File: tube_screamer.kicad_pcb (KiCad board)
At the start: 2 copper layers, 38 x 45 mm, 37 parts, among them Q1 BC817, U1 TL072

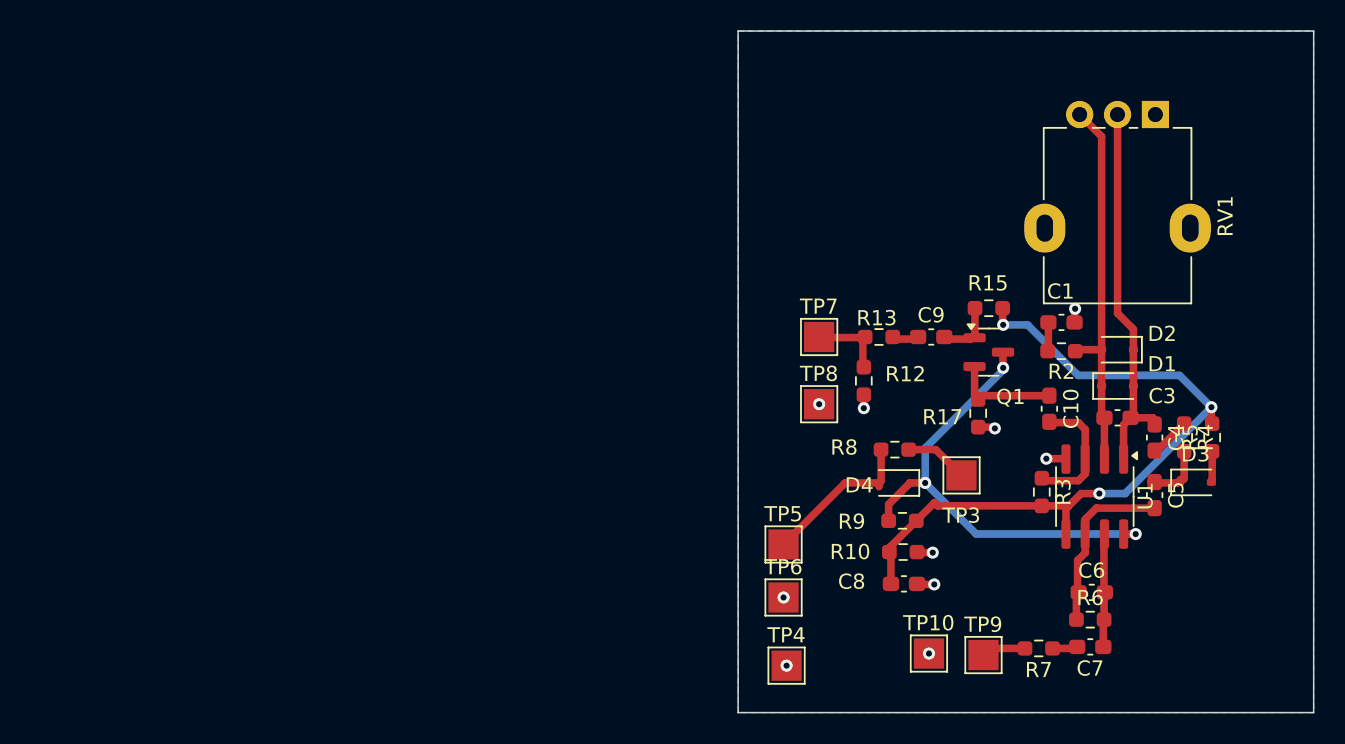
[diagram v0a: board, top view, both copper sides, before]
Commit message: Updated schematic
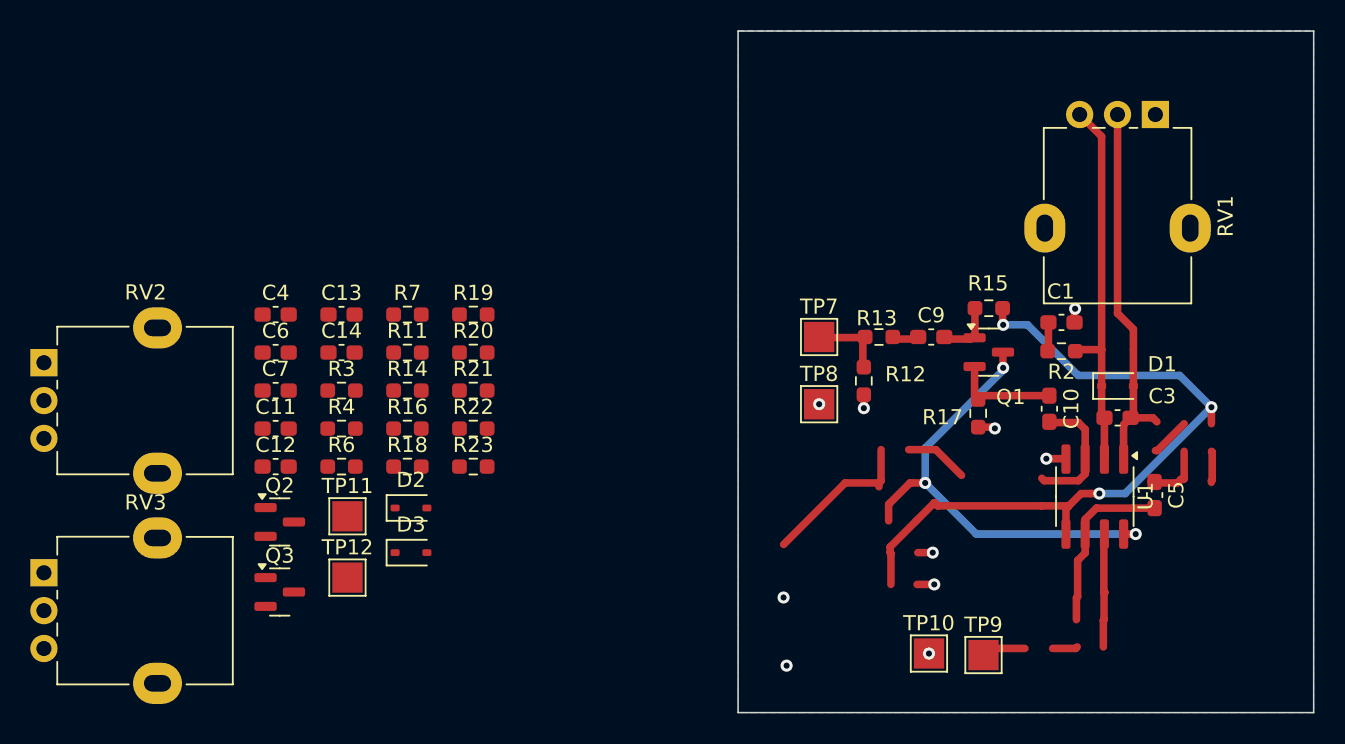
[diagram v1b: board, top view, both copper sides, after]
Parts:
- removed C8: 10u, Capacitor_SMD:C_0603_1608Metric_Pad1.08x0.95mm_HandSolder
- removed D4: 1N4148WS, Diode_SMD:D_SOD-323
- removed R10, R9: 47k, Resistor_SMD:R_0603_1608Metric_Pad0.98x0.95mm_HandSolder
- removed R5: 4.7k, Resistor_SMD:R_0603_1608Metric_Pad0.98x0.95mm_HandSolder
- removed R8: 510, Resistor_SMD:R_0603_1608Metric_Pad0.98x0.95mm_HandSolder
- removed TP3: Red Error LED, TestPoint:TestPoint_Pad_2.0x2.0mm
- removed TP4, TP6: ground, TestPoint:TestPoint_Pad_2.0x2.0mm
- removed TP5: Power Supply, TestPoint:TestPoint_Pad_2.0x2.0mm
- added C11: 10u, Capacitor_SMD:C_0603_1608Metric_Pad1.08x0.95mm_HandSolder, F.Cu at (69.5, 126.2)
- added C12: 100n, Capacitor_SMD:C_0603_1608Metric_Pad1.08x0.95mm_HandSolder, F.Cu at (69.5, 128.8)
- added C13: 10u, Capacitor_SMD:C_0603_1608Metric_Pad1.08x0.95mm_HandSolder, F.Cu at (73.8, 118.7)
- added C14: 10u, Capacitor_SMD:C_0603_1608Metric_Pad1.08x0.95mm_HandSolder, F.Cu at (73.8, 121.2)
- added Q2: MMBT5551, Package_TO_SOT_SMD:SOT-23, F.Cu at (69.7, 132.4)
- added Q3: MMBT5551, Package_TO_SOT_SMD:SOT-23, F.Cu at (69.7, 137.0)
- added R11: 100, Resistor_SMD:R_0603_1608Metric_Pad0.98x0.95mm_HandSolder, F.Cu at (78.2, 121.2)
- added R14: 1k, Resistor_SMD:R_0603_1608Metric_Pad0.98x0.95mm_HandSolder, F.Cu at (78.2, 123.7)
- added R16: 1k, Resistor_SMD:R_0603_1608Metric_Pad0.98x0.95mm_HandSolder, F.Cu at (78.2, 126.2)
- added R18: 1k, Resistor_SMD:R_0603_1608Metric_Pad0.98x0.95mm_HandSolder, F.Cu at (78.2, 128.8)
- added R19: 510k, Resistor_SMD:R_0603_1608Metric_Pad0.98x0.95mm_HandSolder, F.Cu at (82.5, 118.7)
- added R20: 10k, Resistor_SMD:R_0603_1608Metric_Pad0.98x0.95mm_HandSolder, F.Cu at (82.5, 121.2)
- added R21: 10k, Resistor_SMD:R_0603_1608Metric_Pad0.98x0.95mm_HandSolder, F.Cu at (82.5, 123.7)
- added R22: 10k, Resistor_SMD:R_0603_1608Metric_Pad0.98x0.95mm_HandSolder, F.Cu at (82.5, 126.2)
- added R23: 10k, Resistor_SMD:R_0603_1608Metric_Pad0.98x0.95mm_HandSolder, F.Cu at (82.5, 128.8)
- added RV2: 20k, Potentiometer_THT:Potentiometer_Alpha_RD901F-40-00D_Single_Vertical, F.Cu at (54.2, 121.9)
- added RV3: 100k, Potentiometer_THT:Potentiometer_Alpha_RD901F-40-00D_Single_Vertical, F.Cu at (54.2, 135.8)
- added TP11: input, TestPoint:TestPoint_Pad_2.0x2.0mm, F.Cu at (74.2, 132.0)
- added TP12: ground, TestPoint:TestPoint_Pad_2.0x2.0mm, F.Cu at (74.2, 136.1)
- C3: value 51p -> 47p
- C6: value 220p -> 220n
- C7: value 220n -> 1u
- Q1: value BC817 -> MMBT5551
- R12: value 1000k -> 1 Meg
- R15: value 470k -> 510k
- R4: value 10k -> 1k
- R6: value 680k -> 1k
- R7: value 1k -> 220
- TP9: value input -> output
- moved C4 58.6 mm to (69.5, 118.7), turned to 0 degrees
- moved C7 56.4 mm to (69.5, 123.7), turned to 0 degrees
- moved C6 56.2 mm to (69.5, 121.2)
- moved R4 55.6 mm to (73.8, 126.2), turned to 0 degrees
- moved D3 52.0 mm to (78.4, 134.4)
- moved R6 50.5 mm to (73.8, 128.8)
- moved D2 47.8 mm to (78.4, 131.5), turned to 0 degrees
- moved R7 47.2 mm to (78.2, 118.7), turned to 0 degrees
- moved R3 46.7 mm to (73.8, 123.7), turned to 0 degrees
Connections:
- C4 pad 1: Net-(D1-A) -> 0
- C5 pad 1: Net-(D3-K) -> Net-(C4-Pad2)
- C6 pad 1: Net-(U1B--) -> Net-(C6-Pad1)
- C7 pad 1: Net-(C6-Pad2) -> Net-(C7-Pad1)
- R4 pad 2: Net-(D3-K) -> Net-(D1-A)
- R6 pad 1: Net-(U1B--) -> Net-(C7-Pad1)
- R6 pad 2: Net-(C6-Pad2) -> Net-(U1B--)
- R7 pad 1: Net-(C7-Pad2) -> Net-(C6-Pad2)
- R7 pad 2: Net-(R7-Pad2) -> 0
- RV1 pad 1: unconnected-(RV1-Pad1) -> Net-(D1-A)
- TP9 pad 1: Net-(R7-Pad2) -> Net-(C11-Pad2)
- U1 pad 7: Net-(C6-Pad2) -> Net-(C7-Pad1)
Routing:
- net (no net): track 0.00 -> 14.7 mm
- net Net-(D4-A): track 10.5 -> 0.00 mm
- net Net-(C7-Pad1): track 0.00 -> 7.53 mm
- net Net-(C6-Pad2): track 7.53 -> 0.00 mm
- net Net-(R8-Pad1): track 4.19 -> 0.00 mm
- net Net-(D3-K): track 4.14 -> 0.00 mm
- net Net-(C4-Pad2): track 2.64 -> 6.78 mm
- net Net-(R7-Pad2): track 2.92 -> 0.00 mm
- net Net-(C11-Pad2): track 0.00 -> 2.92 mm
